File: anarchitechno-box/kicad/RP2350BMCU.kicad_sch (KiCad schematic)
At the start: 49 parts, among them J2 Conn_01x03_Socket, J4 C2988369, Q201 12mhz, SW1 C318884, U101 <value>, U201 TLV74311PDBVR, U21 C85364, U67 LP5907MFX-3.3

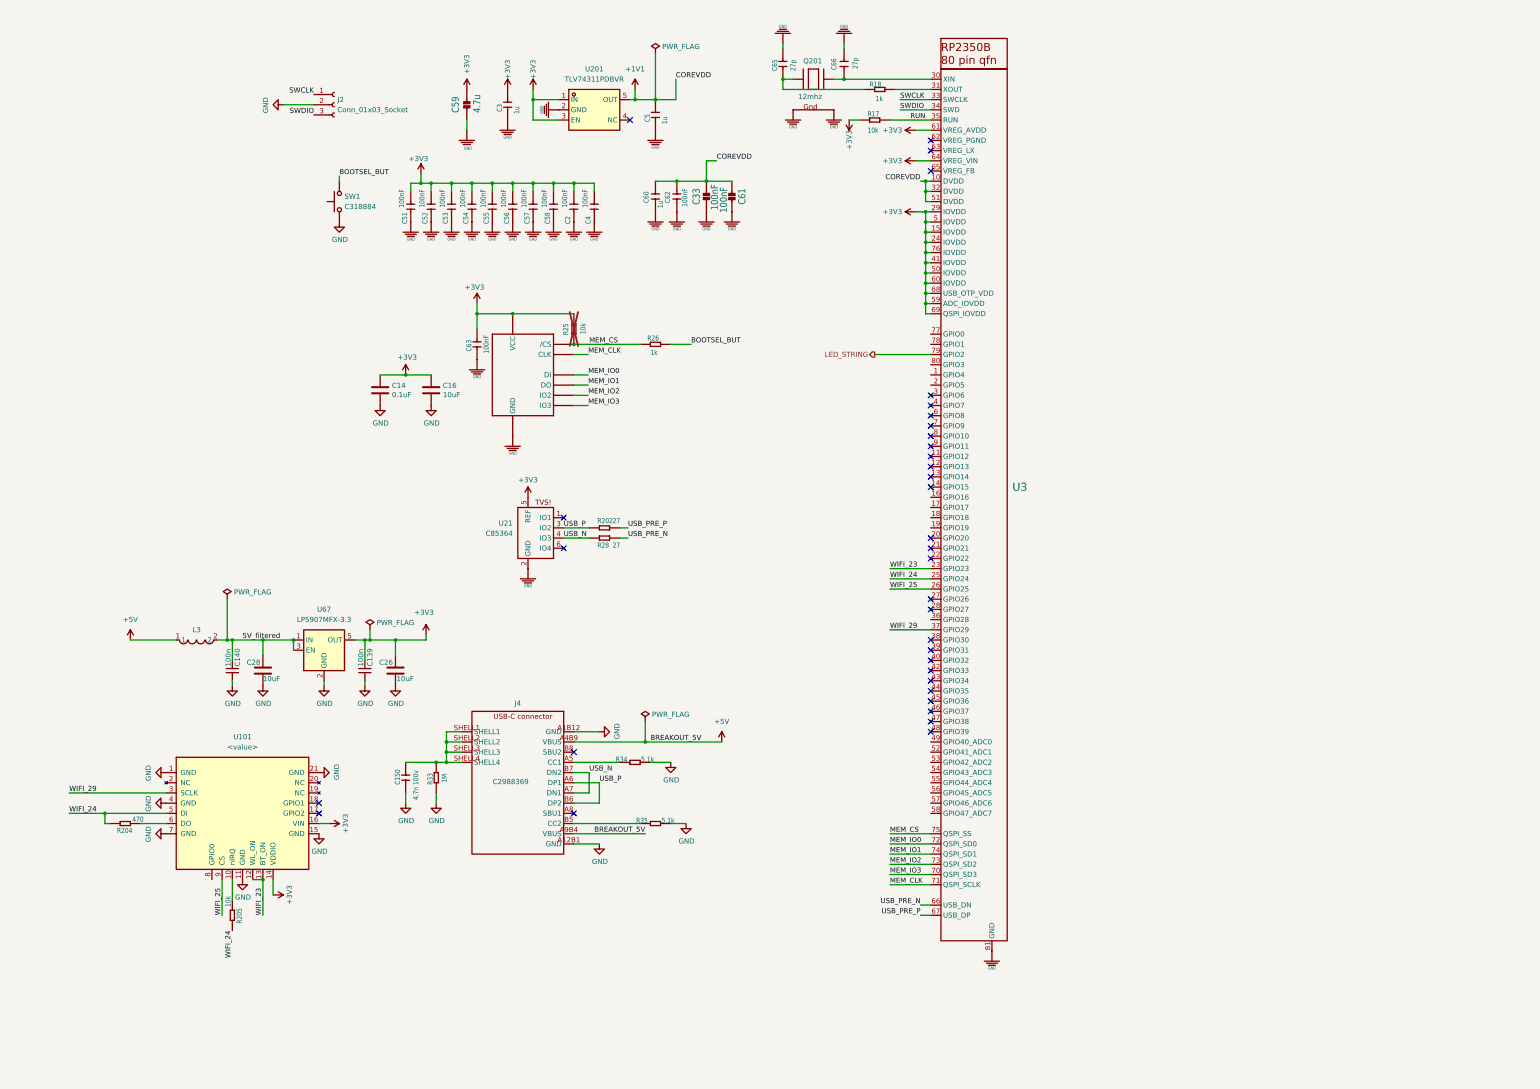
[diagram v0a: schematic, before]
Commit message: Large intermediate schematic push. Remaining todos are on frontpage.
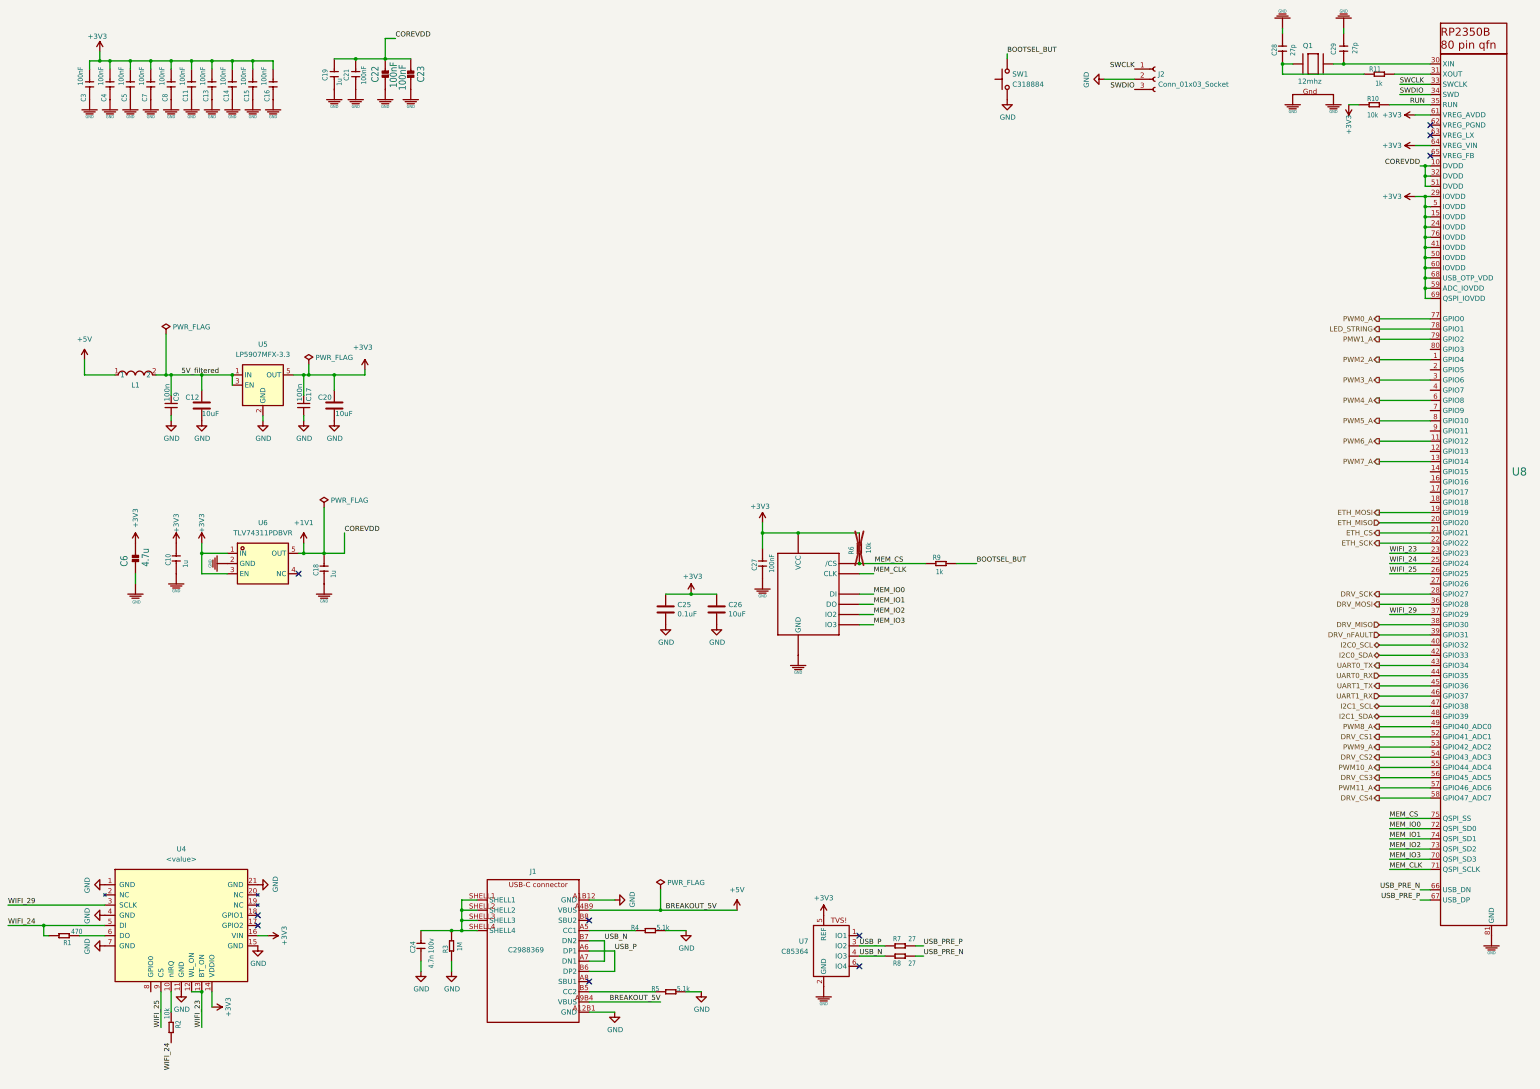
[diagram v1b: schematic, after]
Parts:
- renumbered C3 to C10, C56 to C11, C28 to C12, C57 to C13, C58 to C14, C2 to C15, C4 to C16, C139 to C17, C5 to C18, C60 to C19, C26 to C20, C62 to C21, C33 to C22, C61 to C23, C150 to C24, C14 to C25, C16 to C26, C63 to C27, C65 to C28, C66 to C29, C51 to C3, C52 to C4, C53 to C5, C59 to C6, C54 to C7, C55 to C8, C140 to C9, J4 to J1, L3 to L1, Q201 to Q1, R204 to R1, R17 to R10, R18 to R11, R205 to R2, R33 to R3, R34 to R4, R35 to R5, R25 to R6, R202 to R7, R28 to R8, R26 to R9, U$2 to U$1, U101 to U4, U67 to U5, U201 to U6, U21 to U7, U3 to U8
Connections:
- net LED_STRING: now also U8.78 (GPIO1); no longer U8.79 (GPIO2)
- net PWM2_A: now reaches U8.1 (GPIO4)
- net PWM6_A: now reaches U8.11 (GPIO12)
- net PWM7_A: now reaches U8.13 (GPIO14)
- net ETH_MOSI: now reaches U8.19 (GPIO19)
- net ETH_MISO: now reaches U8.20 (GPIO20)
- net ETH_CS: now reaches U8.21 (GPIO21)
- net ETH_SCK: now reaches U8.22 (GPIO22)
- net DRV_SCK: now reaches U8.28 (GPIO27)
- net PWM3_A: now reaches U8.3 (GPIO6)
- net DRV_MOSI: now reaches U8.36 (GPIO28)
- net DRV_MISO: now reaches U8.38 (GPIO30)
- net DRV_nFAULT: now reaches U8.39 (GPIO31)
- net I2C0_SCL: now reaches U8.40 (GPIO32)
- net I2C0_SDA: now reaches U8.42 (GPIO33)
- net UART0_TX: now reaches U8.43 (GPIO34)
- net UART0_RX: now reaches U8.44 (GPIO35)
- net UART1_TX: now reaches U8.45 (GPIO36)
- net UART1_RX: now reaches U8.46 (GPIO37)
- net I2C1_SCL: now reaches U8.47 (GPIO38)
- net I2C1_SDA: now reaches U8.48 (GPIO39)
- net PWM8_A: now reaches U8.49 (GPIO40_ADC0)
- net DRV_CS1: now reaches U8.52 (GPIO41_ADC1)
- net PWM9_A: now reaches U8.53 (GPIO42_ADC2)
- net DRV_CS2: now reaches U8.54 (GPIO43_ADC3)
- net PWM10_A: now reaches U8.55 (GPIO44_ADC4)
- net DRV_CS3: now reaches U8.56 (GPIO45_ADC5)
- net PWM11_A: now reaches U8.57 (GPIO46_ADC6)
- net DRV_CS4: now reaches U8.58 (GPIO47_ADC7)
- net PWM4_A: now reaches U8.6 (GPIO8)
- net PWM0_A: now reaches U8.77 (GPIO0)
- net PWM5_A: now reaches U8.8 (GPIO10)
- new net PMW1_A: U8.79 (GPIO2)
- no-connect marks 35 -> 10
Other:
- moved on the sheet: C10, C11, C12, C13, C14, C15, C16, C17, C18, C19, C20, C21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
